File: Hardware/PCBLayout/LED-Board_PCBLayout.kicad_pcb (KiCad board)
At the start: 2 copper layers, 9 parts, among them U1 L78L05_TO92

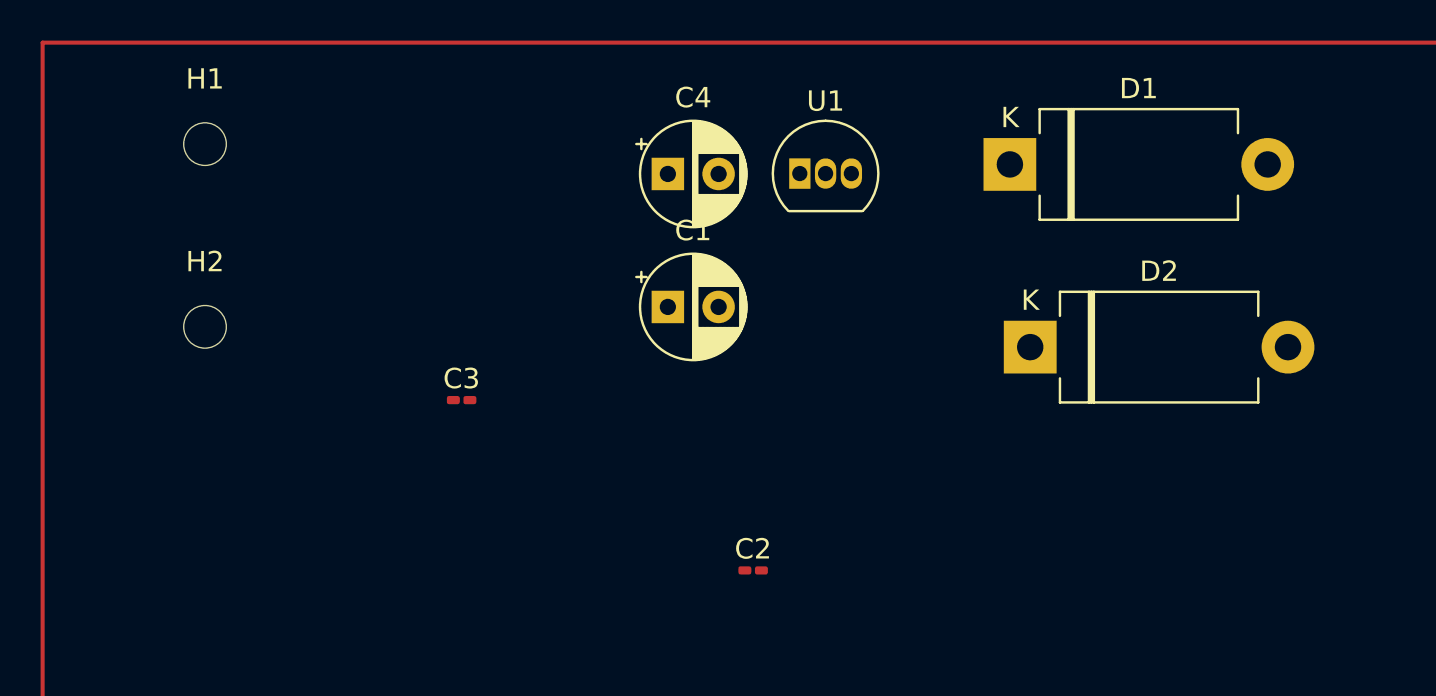
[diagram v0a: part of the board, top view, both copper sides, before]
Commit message: power supply
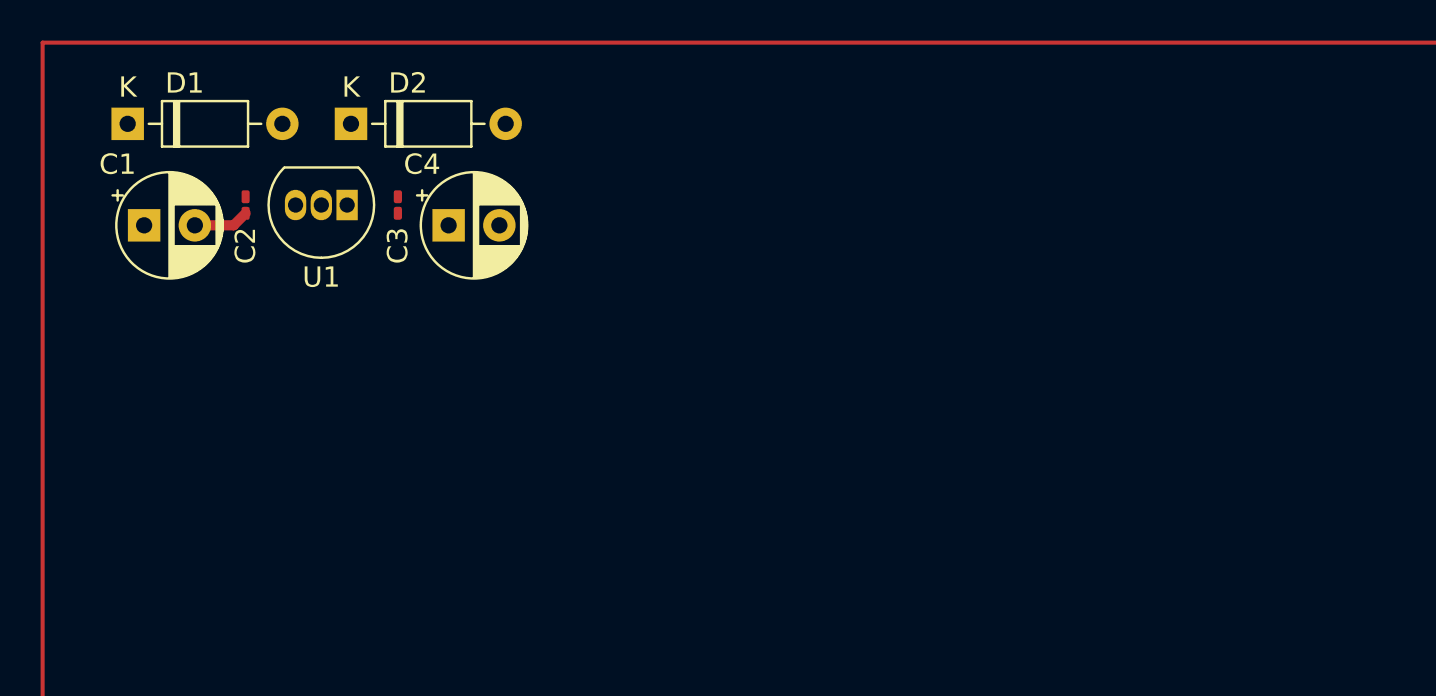
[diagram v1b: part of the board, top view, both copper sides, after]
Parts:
- removed H1, H2: MountingHole_Pad, MountingHole:MountingHole_2.1mm
- D1, D2: footprint Diode_THT:D_DO-201_P12.70mm_Horizontal -> Diode_THT:D_DO-35_SOD27_P7.62mm_Horizontal
- moved D1 43.5 mm to (24.2, 24.0)
- moved D2 35.2 mm to (35.2, 24.0)
- moved C2 30.8 mm to (30.0, 28.0), turned to -90 degrees
- moved C1 26.1 mm to (25.0, 29.0)
- moved U1 22.4 mm to (35.0, 28.0), turned to 180 degrees
- moved C4 11.1 mm to (40.0, 29.0)
- moved C3 10.1 mm to (37.5, 28.0), turned to -90 degrees
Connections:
- U1 pad 2: GND -> unconnected-(U1-Pad2)
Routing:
- net GND: track 0.00 -> 2.75 mm
